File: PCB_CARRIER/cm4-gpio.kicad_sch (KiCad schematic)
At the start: 35 parts, among them J2 Micro_SD_Card_Det2, Q1 BSS138, Q2 BSS138, Q3 BSS138, Q4 BC817-40, SW1 SW_DIP_x04, U4 RT9742GGJ5

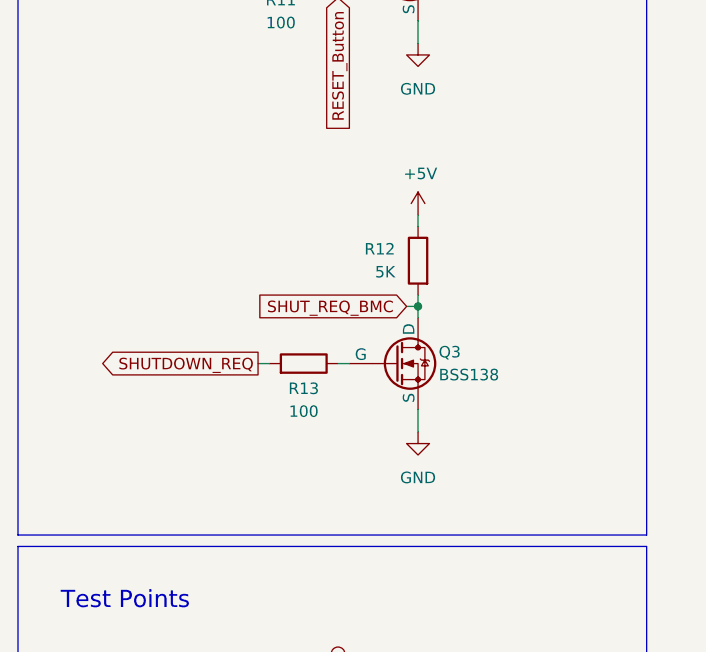
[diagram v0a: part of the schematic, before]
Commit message: fixing the mosfet logic on PMIC_EN
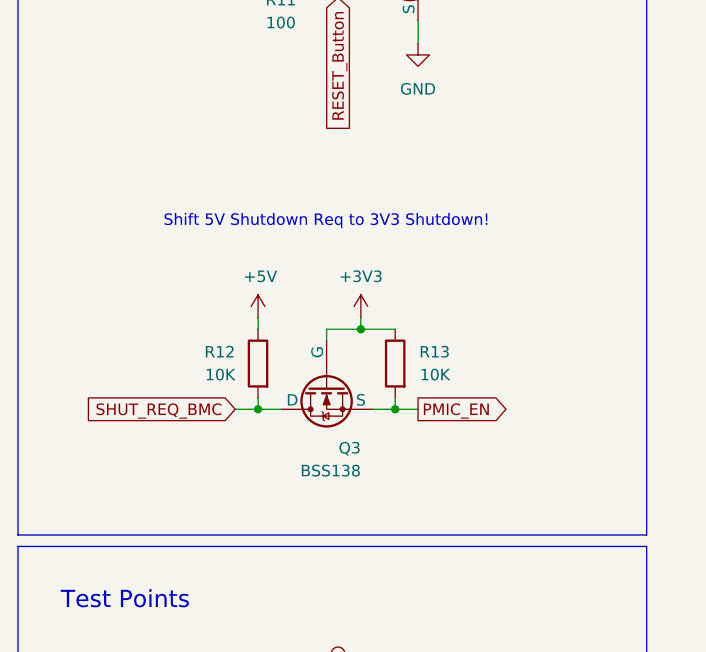
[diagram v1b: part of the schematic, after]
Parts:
- R12: value 5K -> 10K
- R13: value 100 -> 10K
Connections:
- net +3V3: now also Q3.2 (G), R13.1
- net GND: no longer Q3.3 (S)
- net PMIC_EN: now also Q3.3 (S), R13.2
- net SHUTDOWN_REQ: no longer R13.2
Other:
- note added: "Shift 5V Shutdown Req to 3V3 Shutdown!"
- moved on the sheet: Q3, R12
